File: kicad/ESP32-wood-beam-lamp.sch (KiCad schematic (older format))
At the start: 48 parts, among them J1 Screw_Terminal_01x05, J2 Screw_Terminal_01x05, J3 Serial-Prog, J4 Conn_01x02, J5 NextionDisplay, J6 USB_B_Micro, J7 AUX, Q1 IRF3708, Q2 IRF3708, SW1 Flash, SW2 Reset, U1 TLV70233_SOT23-5, U2 ESP-WROOM-32, U3 LevelShifter, U4 BMP280

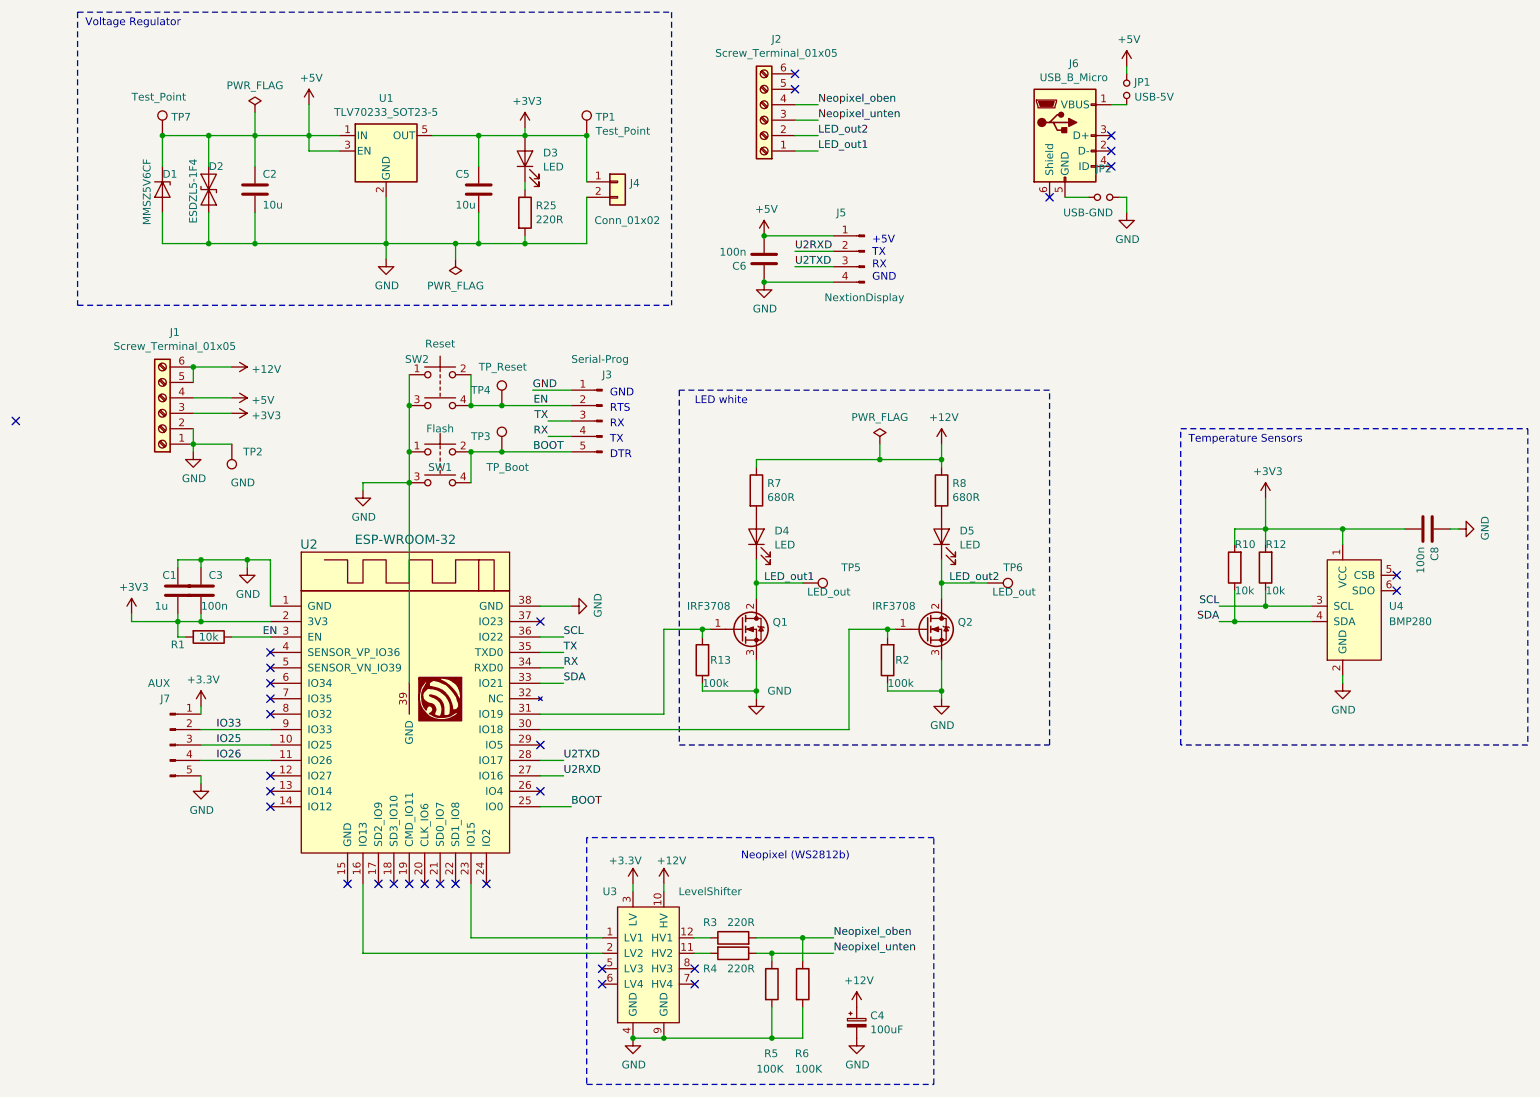
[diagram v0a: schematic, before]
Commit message: rotary Encoder added
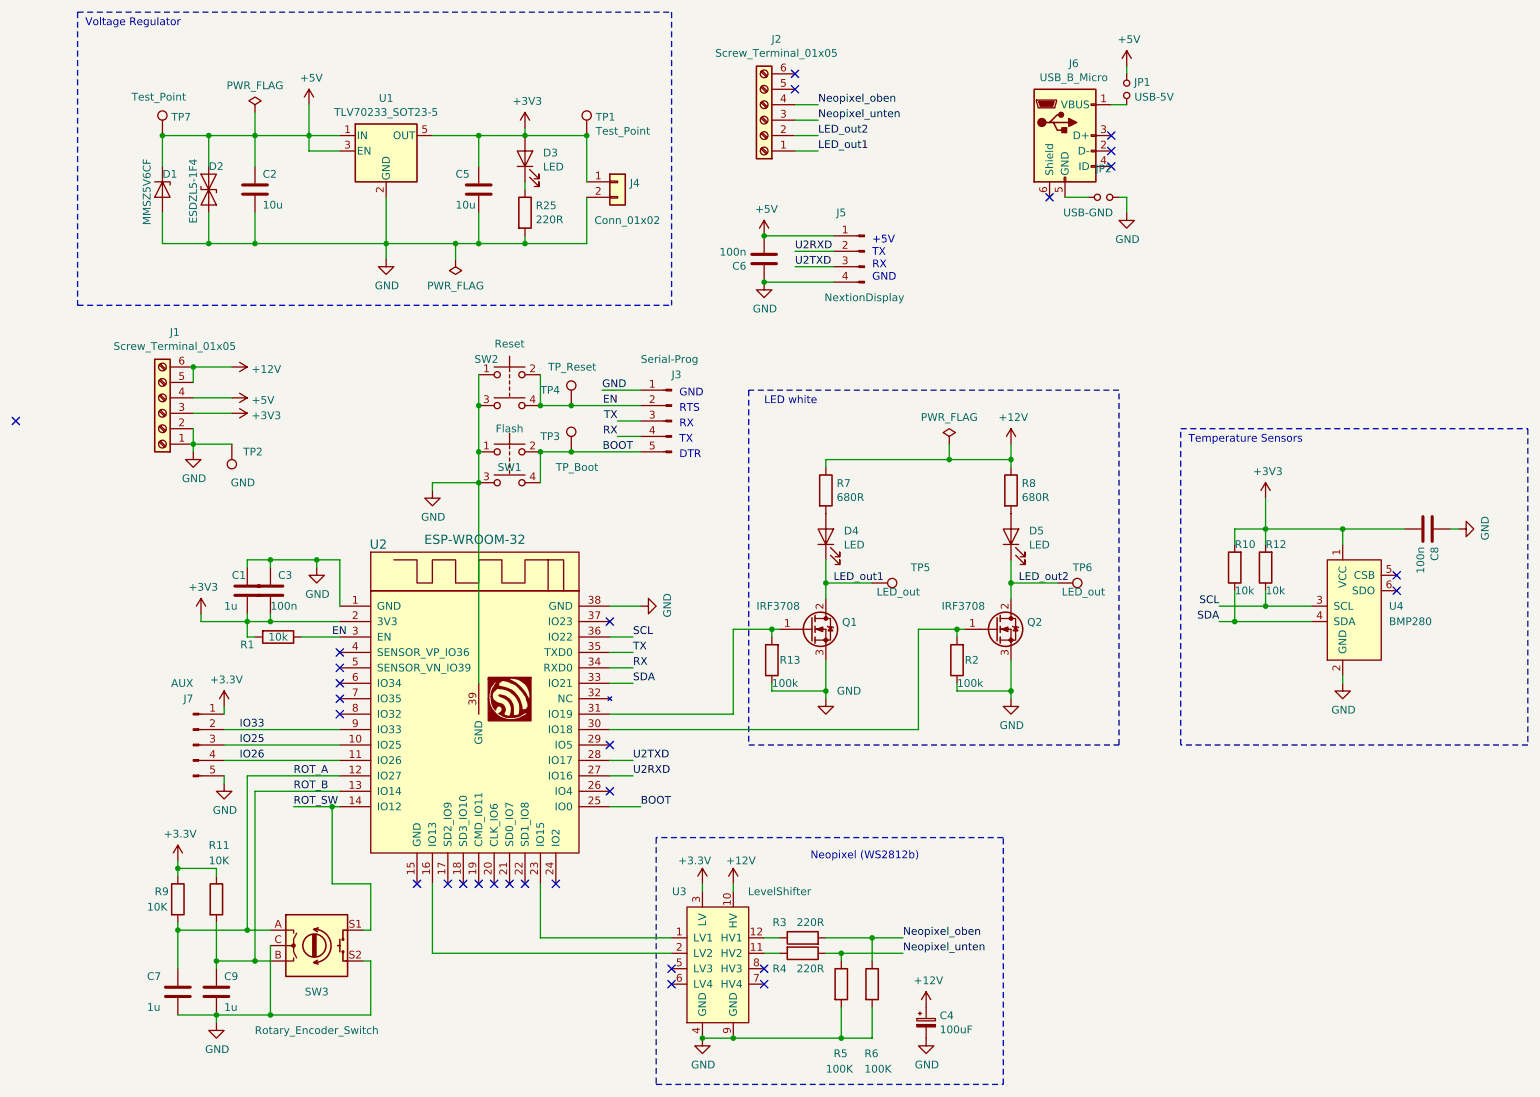
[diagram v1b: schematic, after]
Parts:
- added C7, C9: 1u, symbol Device:C
- added R11, R9: 10K, symbol Device:R
- added SW3: Rotary_Encoder_Switch, symbol Device:Rotary_Encoder_Switch
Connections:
- net +3V3: now also R11.1, R9.1
- net GND: now also C7.2, C9.2, SW3.C, SW3.S2
- net ROT_A: now reaches U2.12 (IO27)
- net ROT_A: now also C7.1, R9.2, SW3.A
- net ROT_B: now reaches U2.13 (IO14)
- net ROT_B: now also C9.1, R11.2, SW3.B
- net ROT_SW: now reaches U2.14 (IO12)
- net ROT_SW: now also SW3.S1
- no-connect marks 32 -> 29
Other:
- moved on the sheet: C1, C3, C4, D4, D5, J3, J7, Q1, Q2, R1, R13, R2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
